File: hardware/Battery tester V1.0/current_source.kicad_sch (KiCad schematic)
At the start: 17 parts, among them K1 Relay_DPDT, Q1 IRF540N, Q2 BC817, U1 LM358

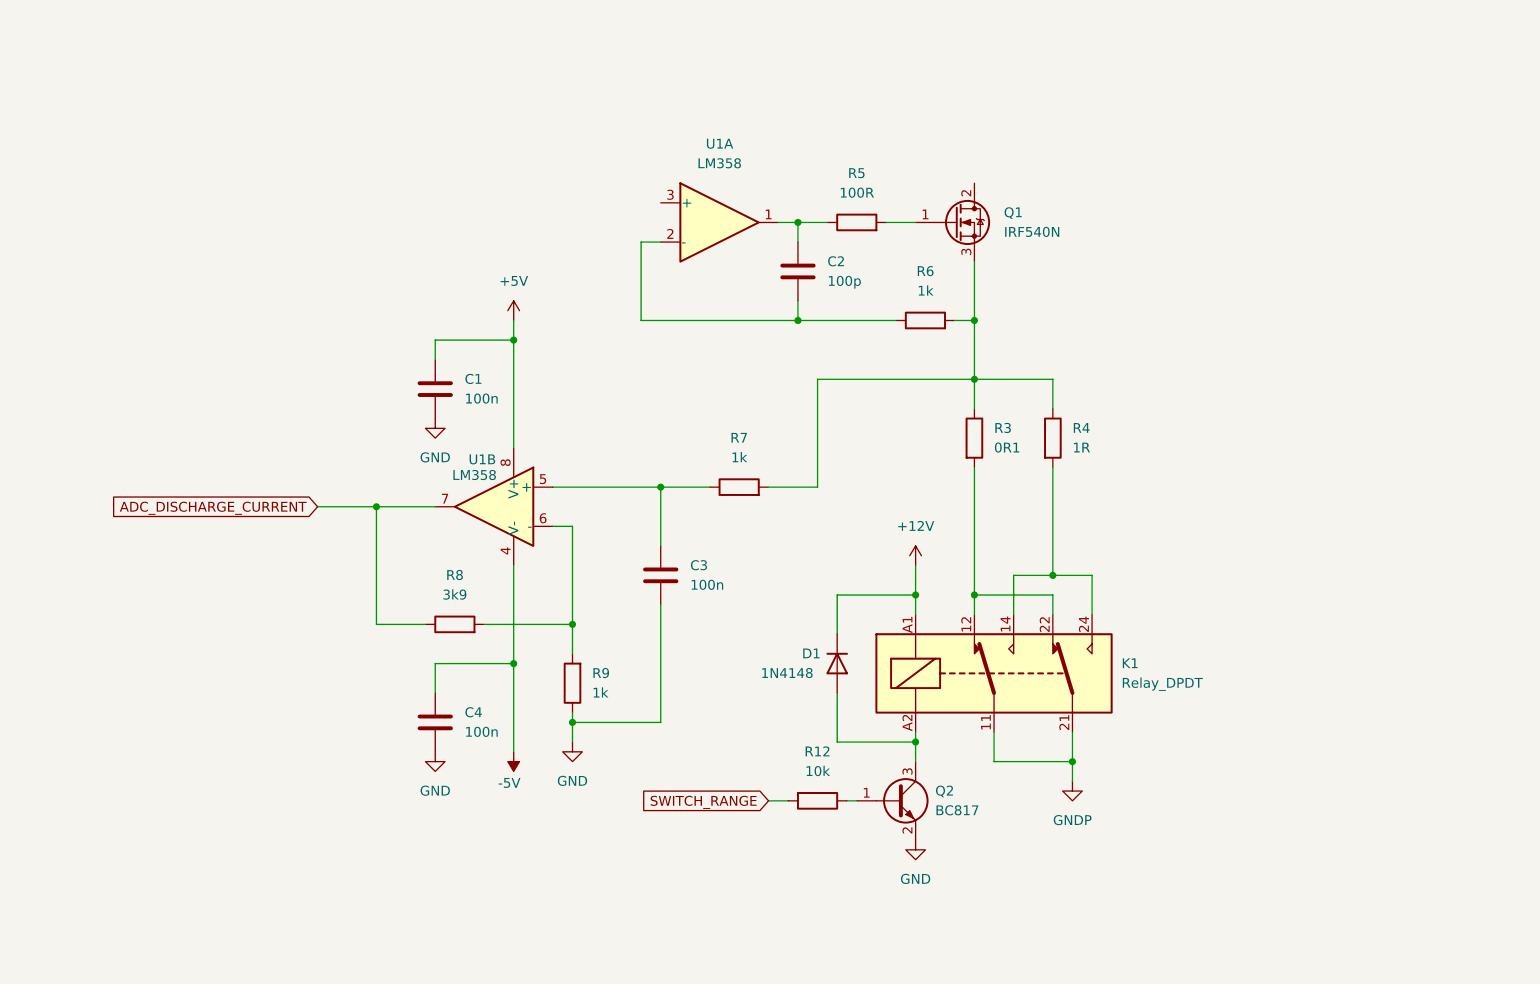
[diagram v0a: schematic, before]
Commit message: update main pcb schematic
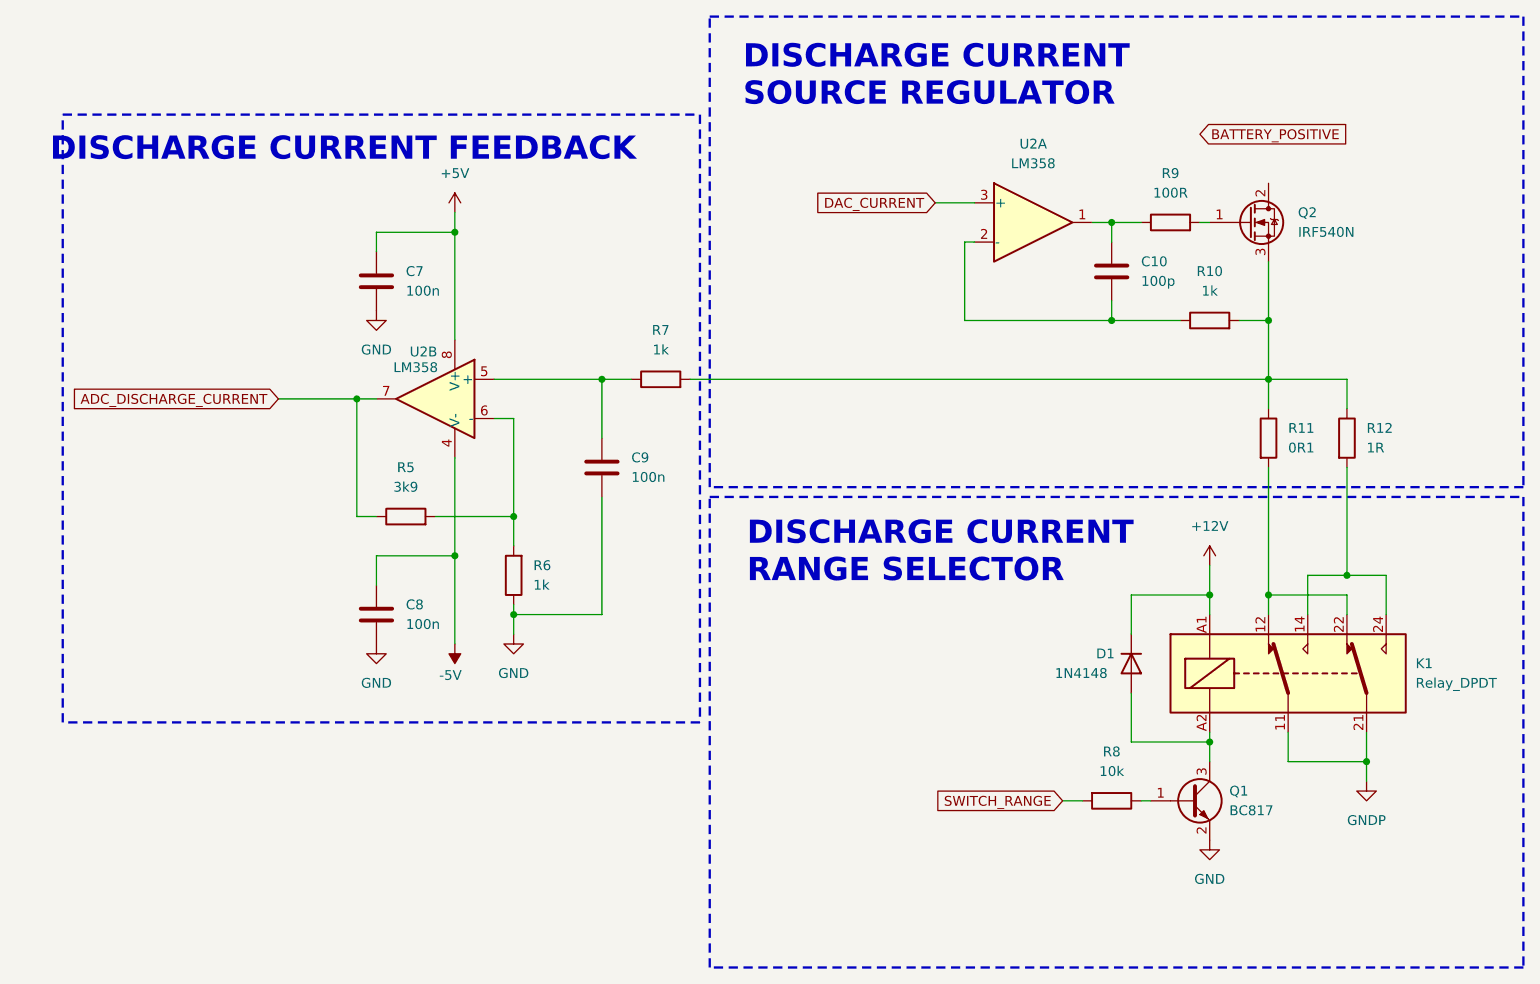
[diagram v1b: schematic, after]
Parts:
- C10: renamed from C2; footprint (none) -> Capacitor_SMD:C_0805_2012Metric_Pad1.18x1.45mm_HandSolder
- C9: renamed from C3; footprint (none) -> Capacitor_SMD:C_0805_2012Metric_Pad1.18x1.45mm_HandSolder
- R10: renamed from R6; footprint (none) -> Capacitor_SMD:C_0805_2012Metric_Pad1.18x1.45mm_HandSolder
- R11: renamed from R3; footprint (none) -> Capacitor_SMD:C_0805_2012Metric_Pad1.18x1.45mm_HandSolder
- R12: renamed from R4; footprint (none) -> Capacitor_SMD:C_0805_2012Metric_Pad1.18x1.45mm_HandSolder
- R5: renamed from R8; footprint (none) -> Capacitor_SMD:C_0805_2012Metric_Pad1.18x1.45mm_HandSolder
- R6: renamed from R9; footprint (none) -> Capacitor_SMD:C_0805_2012Metric_Pad1.18x1.45mm_HandSolder
- R7: footprint (none) -> Capacitor_SMD:C_0805_2012Metric_Pad1.18x1.45mm_HandSolder
- R8: renamed from R12; footprint (none) -> Capacitor_SMD:C_0805_2012Metric_Pad1.18x1.45mm_HandSolder
- R9: renamed from R5; footprint (none) -> Capacitor_SMD:C_0805_2012Metric_Pad1.18x1.45mm_HandSolder
- U2: renamed from U1; footprint (none) -> Package_SO:SO-8_3.9x4.9mm_P1.27mm
- renumbered C1 to C7, C4 to C8, Q2 to Q1, Q1 to Q2
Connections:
- net DAC_CURRENT: now reaches U2.3 (+)
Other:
- note added: "DISCHARGE CURRENT FEEDBACK"
- note added: "DISCHARGE CURRENT RANGE SELECTOR"
- note added: "DISCHARGE CURRENT SOURCE REGULATOR"
- moved on the sheet: C10, C7, C8, C9, D1, K1, Q1, Q2, R10, R11, R12, R5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
